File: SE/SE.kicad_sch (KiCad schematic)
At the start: 12 parts, among them J1 RJ45, J2 Conn_01x04_Female, J3 Conn_01x03_Female, Q4 BC548

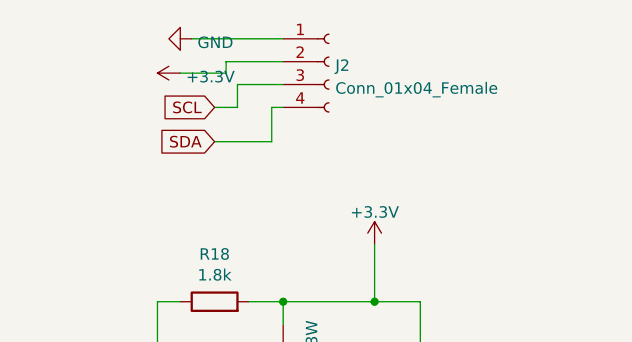
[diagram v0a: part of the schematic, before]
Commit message: PCB Primer Ajuste
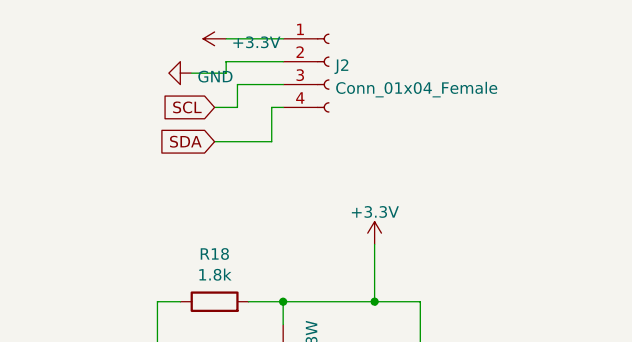
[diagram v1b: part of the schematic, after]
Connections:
- net +3.3V: now also J2.1 (Pin_1); no longer J2.2 (Pin_2)
- net GND: now also J2.2 (Pin_2); no longer J2.1 (Pin_1)
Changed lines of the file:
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@@
+    (stroke (width 0) (type default) (color 0 0 0 0))
+  )
+  (wire (pts (xy 123.19 27.94) (xy 116.84 27.94))
     (stroke (width 0) (type default) (color 0 0 0 0))
   )
@@
     (stroke (width 0) (type default) (color 0 0 0 0))
   )
-  (wire (pts (xy 116.84 29.21) (xy 116.84 27.94))
-    (stroke (width 0) (type default) (color 0 0 0 0))
-  )
   (wire (pts (xy 215.9 49.53) (xy 212.09 49.53))
     (stroke (width 0) (type default) (color 0 0 0 0))
@@
     (stroke (width 0) (type default) (color 0 0 0 0))
   )
-  (wire (pts (xy 111.76 29.21) (xy 116.84 29.21))
-    (stroke (width 0) (type default) (color 0 0 0 0))
-  )
   (wire (pts (xy 138.43 71.12) (xy 123.19 71.12))
     (stroke (width 0) (type default) (color 0 0 0 0))
   )
-  (wire (pts (xy 116.84 27.94) (xy 123.19 27.94))
-    (stroke (width 0) (type default) (color 0 0 0 0))
-  )
   (wire (pts (xy 121.92 36.83) (xy 121.92 33.02))
     (stroke (width 0) (type default) (color 0 0 0 0))
@@
     (stroke (width 0) (type default) (color 0 0 0 0))
   )
+  (wire (pts (xy 116.84 29.21) (xy 113.03 29.21))
+    (stroke (width 0) (type default) (color 0 0 0 0))
+  )
   (wire (pts (xy 214.63 45.72) (xy 212.09 45.72))
     (stroke (width 0) (type default) (color 0 0 0 0))
   )
-  (wire (pts (xy 113.03 25.4) (xy 123.19 25.4))
-    (stroke (width 0) (type default) (color 0 0 0 0))
-  )
   (wire (pts (xy 128.27 97.79) (xy 128.27 102.87))
     (stroke (width 0) (type default) (color 0 0 0 0))
@@
     (stroke (width 0) (type default) (color 0 0 0 0))
   )
+  (wire (pts (xy 116.84 25.4) (xy 123.19 25.4))
+    (stroke (width 0) (type default) (color 0 0 0 0))
+  )
   (wire (pts (xy 215.9 53.34) (xy 217.17 53.34))
     (stroke (width 0) (type default) (color 0 0 0 0))
@@
   )
   (wire (pts (xy 173.99 91.44) (xy 173.99 95.25))
+    (stroke (width 0) (type default) (color 0 0 0 0))
+  )
+  (wire (pts (xy 116.84 27.94) (xy 116.84 29.21))
     (stroke (width 0) (type default) (color 0 0 0 0))
   )
@@
     (pin "8")
   )
-  (symbol (lib_id "power:GND") (at 113.03 25.4 270) (unit 1)
-    (in_bom yes) (on_board yes) (fields_autoplaced)
-    (property "Reference" "#PWR0109" (id 0) (at 106.68 25.4 0)
-      (effects (font (size 1.27 1.27)) hide)
-    )
-    (property "Value" "GND" (id 1) (at 113.665 25.8338 90)
-      (effects (font (size 1.27 1.27)) (justify left))
-    )
-    (property "Footprint" "" (id 2) (at 113.03 25.4 0)
-      (effects (font (size 1.27 1.27)) hide)
-    )
-    (property "Datasheet" "" (id 3) (at 113.03 25.4 0)
+  (symbol (lib_id "power:GND") (at 113.03 29.21 270) (unit 1)
+    (in_bom yes) (on_board yes) (fields_autoplaced)
+    (property "Reference" "#PWR0109" (id 0) (at 106.68 29.21 0)
+      (effects (font (size 1.27 1.27)) hide)
+    )
+    (property "Value" "GND" (id 1) (at 113.665 29.6438 90)
+      (effects (font (size 1.27 1.27)) (justify left))
+    )
+    (property "Footprint" "" (id 2) (at 113.03 29.21 0)
+      (effects (font (size 1.27 1.27)) hide)
+    )
+    (property "Datasheet" "" (id 3) (at 113.03 29.21 0)
       (effects (font (size 1.27 1.27)) hide)
     )
@@
     (pin "2")
   )
-  (symbol (lib_id "power:+3.3V") (at 111.76 29.21 90) (unit 1)
-    (in_bom yes) (on_board yes) (fields_autoplaced)
-    (property "Reference" "#PWR0108" (id 0) (at 115.57 29.21 0)
-      (effects (font (size 1.27 1.27)) hide)
-    )
-    (property "Value" "+3.3V" (id 1) (at 112.395 29.6438 90)
+  (symbol (lib_id "power:+3.3V") (at 116.84 25.4 90) (unit 1)
+    (in_bom yes) (on_board yes) (fields_autoplaced)
+    (property "Reference" "#PWR0108" (id 0) (at 120.65 25.4 0)
+      (effects (font (size 1.27 1.27)) hide)
+    )
+    (property "Value" "+3.3V" (id 1) (at 117.475 25.8338 90)
       (effects (font (size 1.27 1.27)) (justify right))
     )
-    (property "Footprint" "" (id 2) (at 111.76 29.21 0)
-      (effects (font (size 1.27 1.27)) hide)
-    )
-    (property "Datasheet" "" (id 3) (at 111.76 29.21 0)
-      (effects (font (size 1.27 1.27)) hide)
-    )
+    (property "Footprint" "" (id 2) (at 116.84 25.4 0)
+      (effects (font (size 1.27 1.27)) hide)
+    )
+    (property "Datasheet" "" (id 3) (at 116.84 25.4 0)
+      (effects (font (size 1.27 1.27)) hide)
+    )
